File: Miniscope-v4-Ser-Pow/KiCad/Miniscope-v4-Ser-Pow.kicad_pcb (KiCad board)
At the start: 6 copper layers, 9.1 x 12.5 mm, 39 parts, among them J16 Conn_01x20_Female, U1 DS90UB933-Q1, U3 TLV7103318DSER

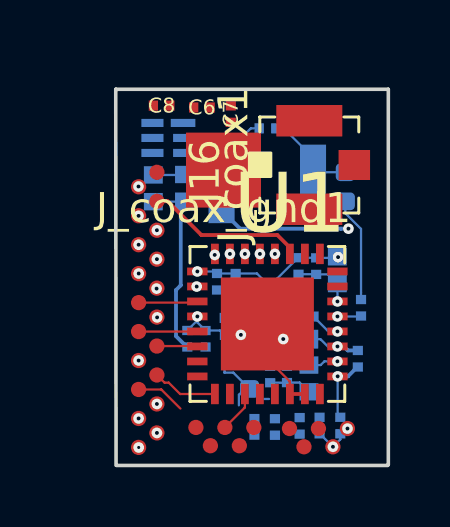
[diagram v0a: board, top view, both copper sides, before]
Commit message: Almost done
- Everything is connected
- All pads are the same
- Traces are as big as possible

To do

- Final check
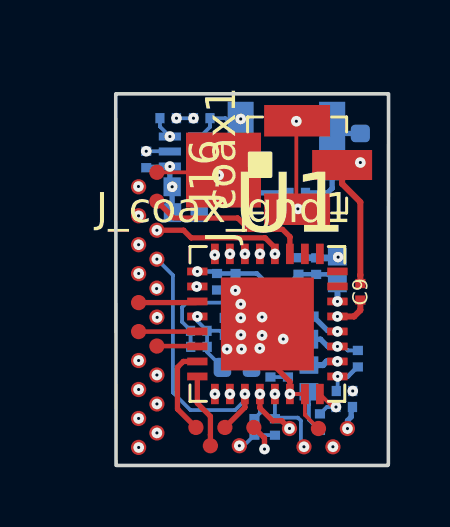
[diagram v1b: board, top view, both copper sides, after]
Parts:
- C6, C7, C8: moved to B.Cu
- C9: moved to F.Cu
- moved R1 2.37 mm to (120.2, 43.3)
- moved C8 1.87 mm to (115.2, 42.2), turned to 270 degrees
- moved R3 1.61 mm to (121.8, 50.5), turned to 180 degrees
- moved L1 1.56 mm to (119.9, 41.6)
- moved L2 1.39 mm to (122.4, 41.8)
- moved C5 1.36 mm to (116.5, 44.0), turned to 180 degrees
- moved C6 1.18 mm to (115.9, 40.8), turned to 0 degrees
- moved C11 1.16 mm to (121.8, 49.9), turned to 0 degrees
- moved C7 0.98 mm to (117.1, 40.8), turned to 180 degrees
- moved U3 0.74 mm to (116.5, 42.0)
- moved C9 0.53 mm to (122.4, 46.6)
- moved L4 0.48 mm to (118.2, 49.1), turned to 180 degrees
- moved C30 0.47 mm to (117.0, 47.9), turned to 180 degrees
- moved J_coax1 0.41 mm to (120.2, 42.4)
- moved C29 0.35 mm to (117.0, 48.5), turned to 180 degrees
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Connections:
- J16 pad 19: VDDD -> +3V3
- J_extra2 pad 3: +5V -> GND
- J_extra2 pad 4: GND -> +5V
- U1 pad : (no net) -> GND
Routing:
- net +3V3: track 6.23 -> 18.8 mm, vias 0 -> 3
- net +5V: track 15.0 -> 27.0 mm, vias 2 -> 3
- net I2C_SDA: track 1.86 -> 8.97 mm, vias 0 -> 3
- net I2C_SCL: track 0.46 -> 6.72 mm, vias 1 -> 3
- net GND: track 22.7 -> 28.3 mm, vias 5 -> 22
- net DIN10: track 0.00 -> 3.00 mm
- net DIN11: track 0.00 -> 2.49 mm
- net CLK_OUT: track 6.74 -> 9.04 mm, vias 1 -> 2
- net VDDD: track 10.9 -> 9.56 mm
- net MODE: track 0.00 -> 1.34 mm, vias 0 -> 1
- net PDB: track 2.20 -> 1.41 mm
- net DOUT_P: track 3.49 -> 4.20 mm, vias 0 -> 1
- net DIN0: track 5.28 -> 5.86 mm
- net FV: track 3.97 -> 3.81 mm, vias 1 -> 2
- net LV: track 2.20 -> 2.27 mm, vias 0 -> 2
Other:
- board size 9.1 x 12.5 mm -> 9.1 x 12.4 mm
